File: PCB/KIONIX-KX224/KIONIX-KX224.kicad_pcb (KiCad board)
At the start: 2 copper layers, 25 x 9 mm, 7 parts, among them J1 Conn_02x03_Odd_Even

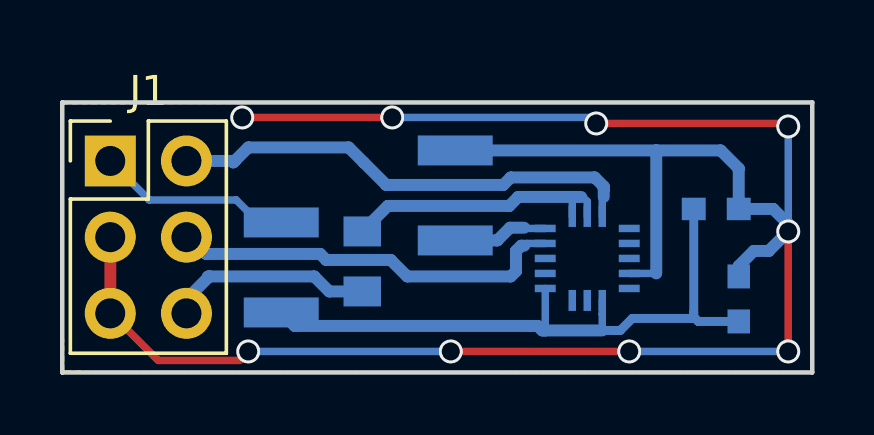
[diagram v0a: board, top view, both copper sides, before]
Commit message: PCB - KX224 V2.0 verified
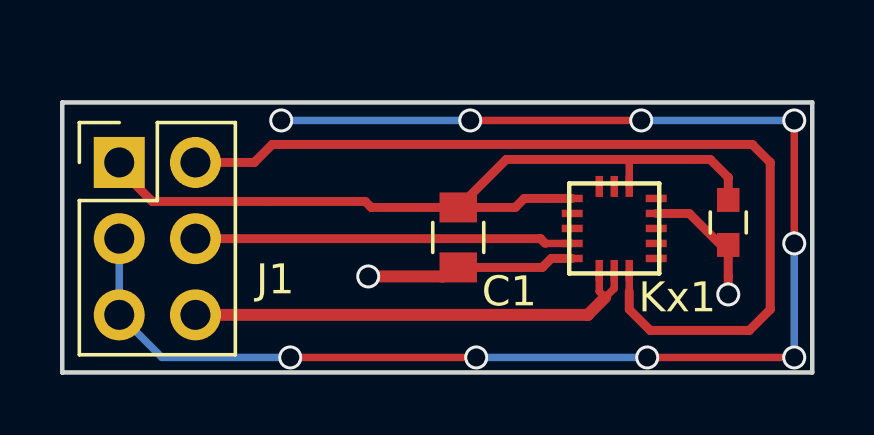
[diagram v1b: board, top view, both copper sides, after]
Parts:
- removed JP1: Jumper, Capacitors_SMD:C_0805
- removed JP2, JP3: Jumper, Capacitors_SMD:C_1210
- C1: footprint Capacitors_SMD:C_0603 -> Capacitors_SMD:C_0805; moved to F.Cu
- C2, Kx1: moved to F.Cu
- moved C1 8.65 mm to (140.2, 94.5), turned to 270 degrees
- moved C2 2.57 mm to (149.2, 94.0), turned to 270 degrees
- moved Kx1 1.35 mm to (145.4, 94.2)
- moved J1 0.30 mm to (128.9, 92.0)
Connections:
- J1 pad 1: Net-(J1-Pad1) -> /VDD
- J1 pad 6: Net-(J1-Pad6) -> /Miso/Mosi
- Kx1 pad 5: Net-(JP3-Pad2) -> GNDREF
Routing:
- net /CS/SCL: track 16.0 -> 31.1 mm
- net GNDREF: track 72.6 -> 62.6 mm, vias 9 -> 11
- net Net-(J1-Pad6): track 6.90 -> 0.00 mm
- net /Miso/Mosi: track 9.19 -> 15.9 mm
- net Net-(J1-Pad1): track 6.55 -> 0.00 mm
- net /VDD: track 22.7 -> 28.1 mm
- net Net-(JP3-Pad2): track 3.19 -> 0.00 mm
- net /SCLK: track 13.4 -> 12.6 mm
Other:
- board text added: "KX224 Eval Board CHAMP - October/2018"
- board text added: "Mosi Miso SCL"
- board text added: "SCLK"
- board text added: "VDD"
